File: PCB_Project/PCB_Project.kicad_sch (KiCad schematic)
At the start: 7 parts

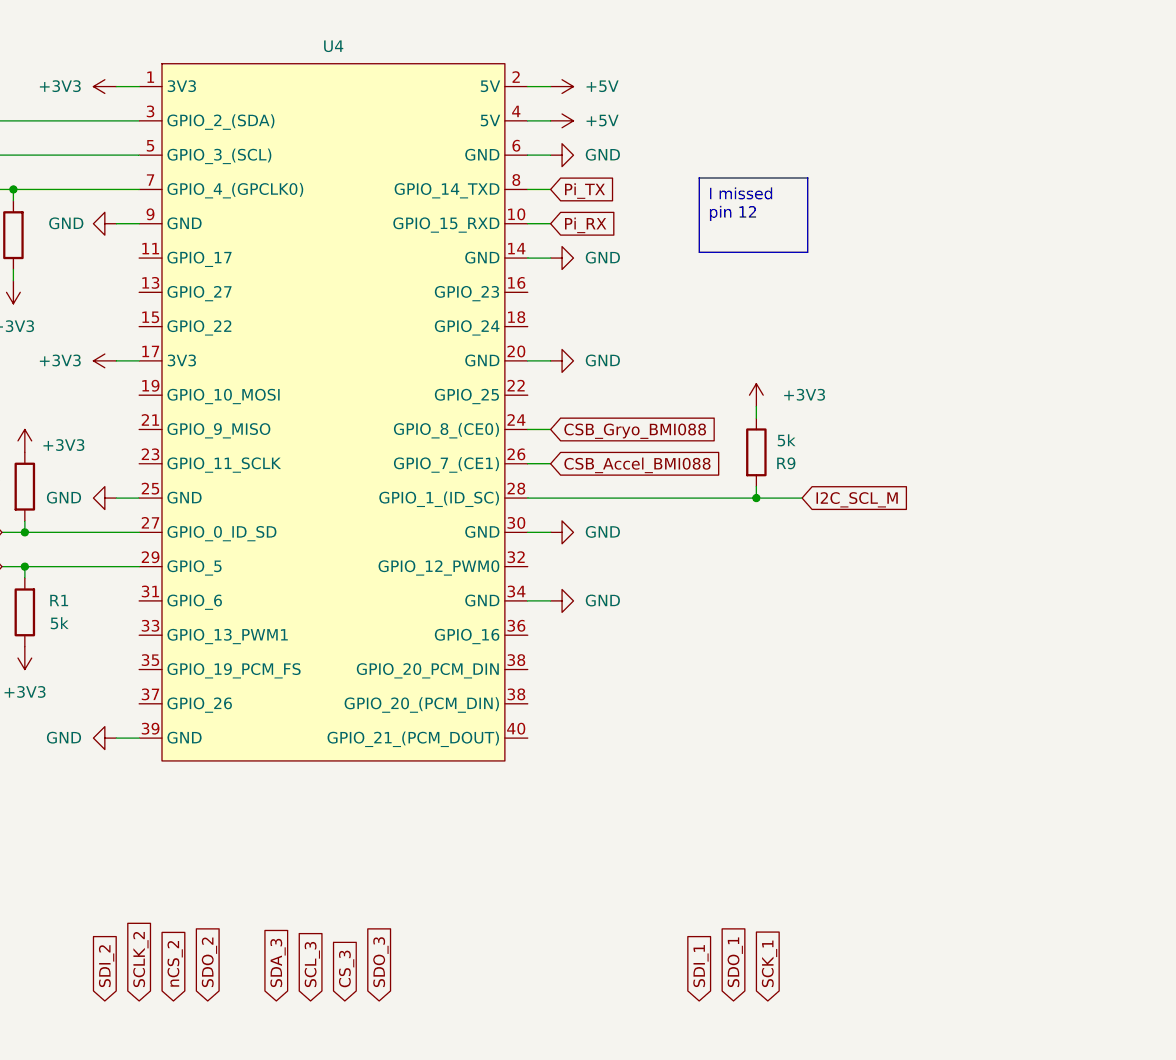
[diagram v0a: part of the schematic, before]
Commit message: more cleaning up and adding footprints
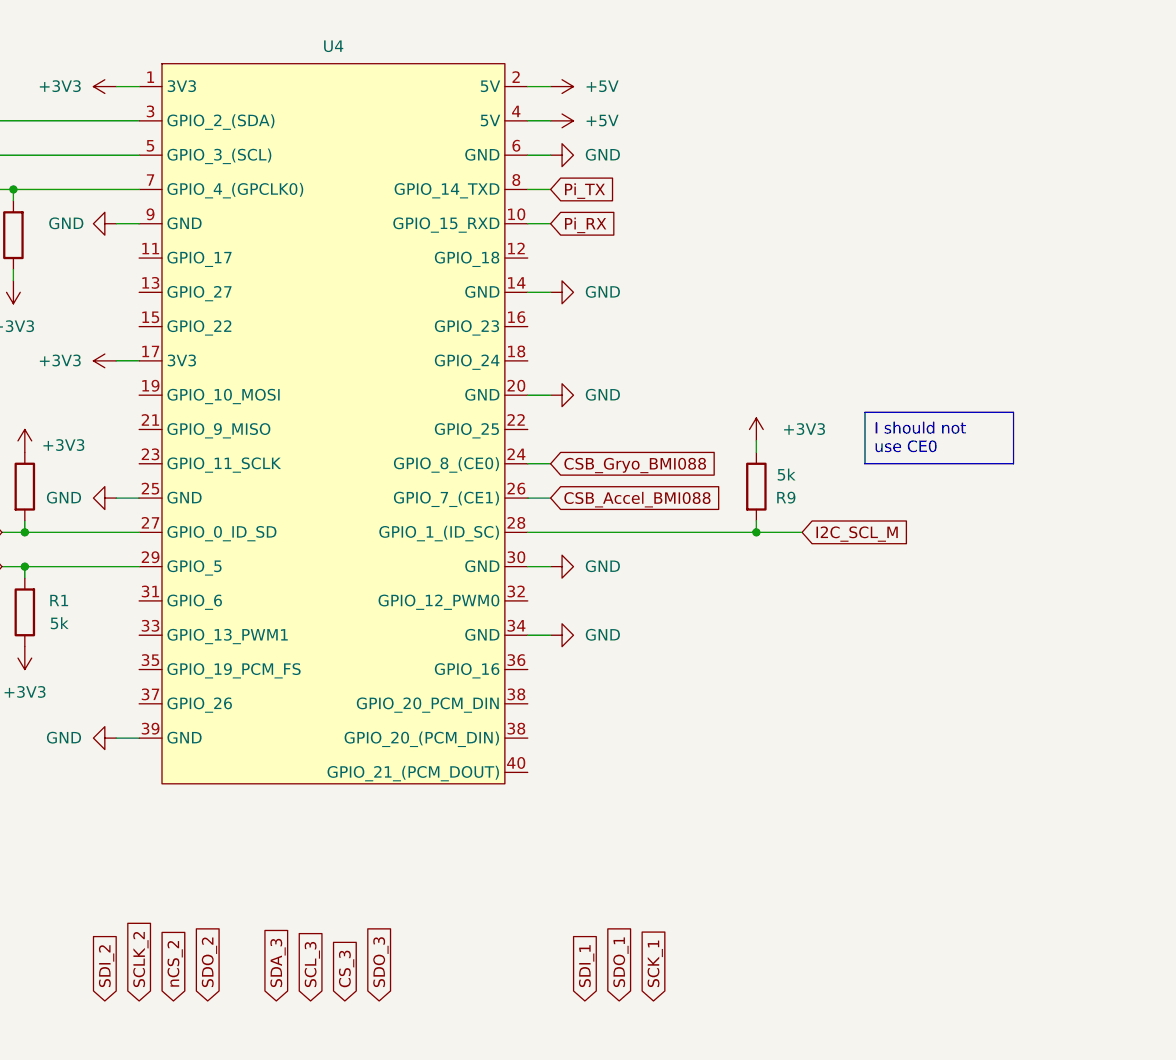
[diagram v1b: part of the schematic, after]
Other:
- moved on the sheet: R9

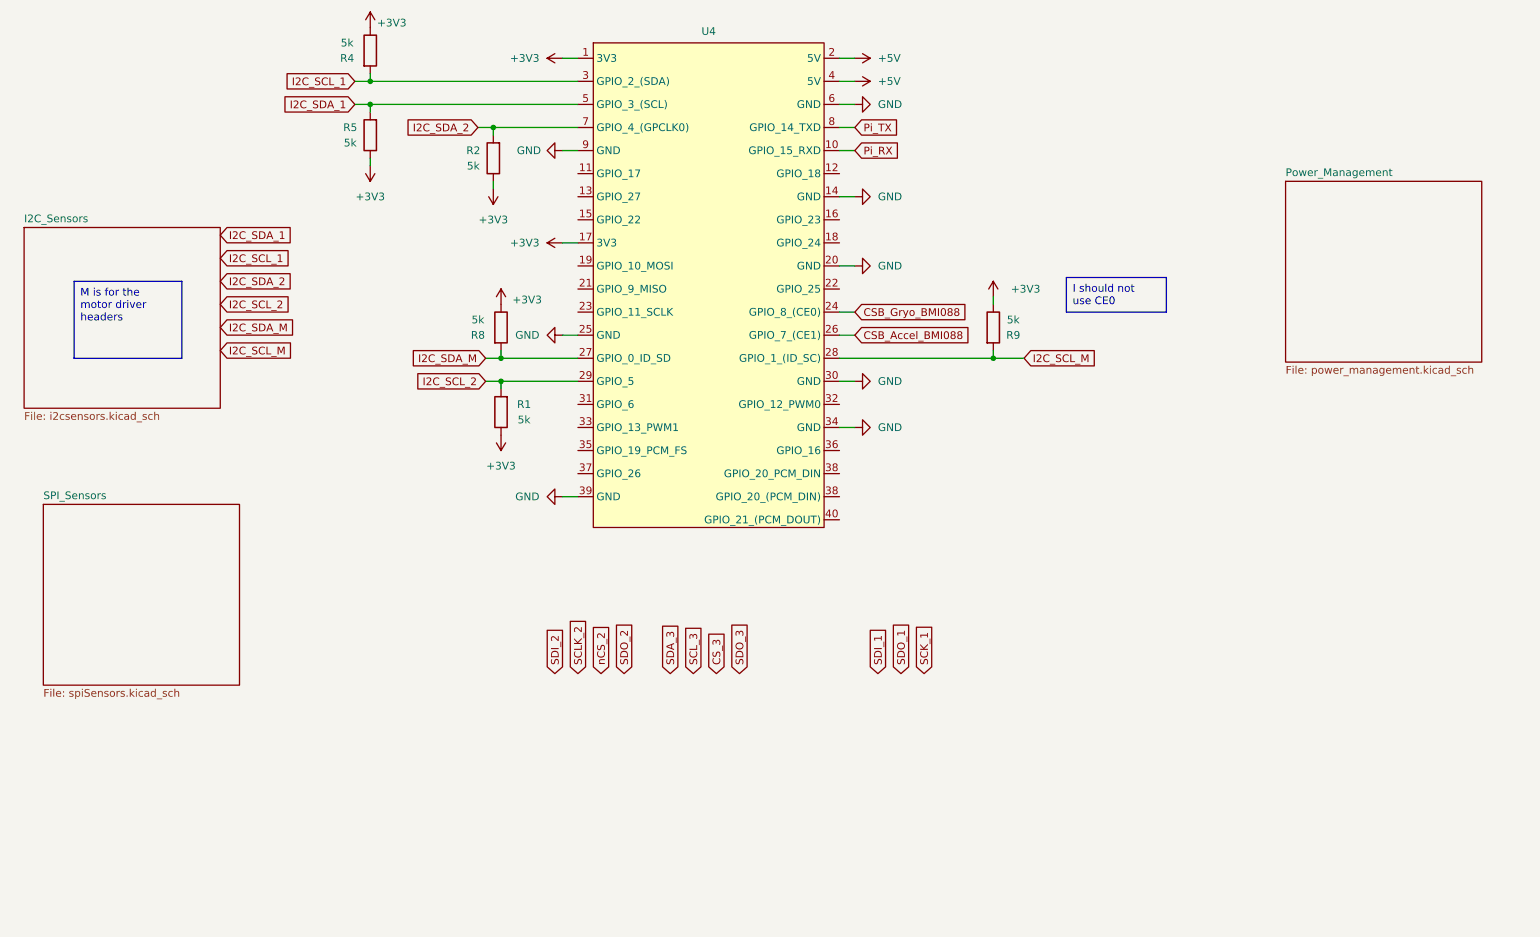
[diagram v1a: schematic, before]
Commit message: need to fix the one damn footprint
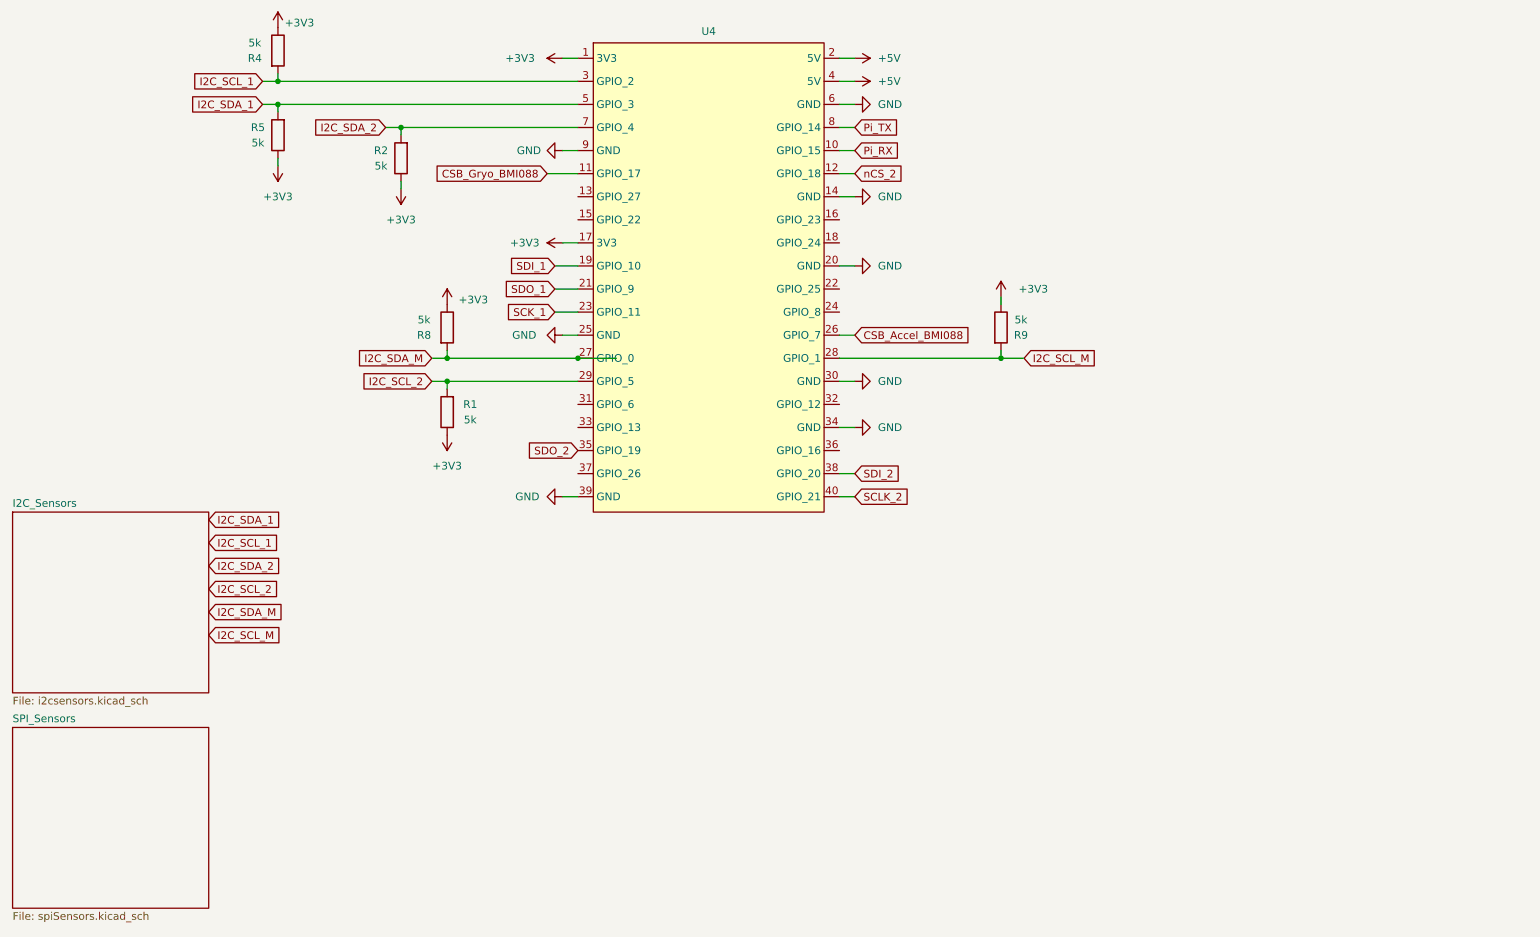
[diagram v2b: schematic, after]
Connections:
- net CSB_Gryo_BMI088: now also U4.11 (GPIO_17); no longer U4.24 (GPIO_8_(CE0))
- net SCK_1: now also U4.23 (GPIO_11)
- net SCLK_2: now also U4.40 (GPIO_21)
- net SDI_1: now also U4.19 (GPIO_10)
- net SDI_2: now also U4.38 (GPIO_20)
- net SDO_1: now also U4.21 (GPIO_9)
- net SDO_2: now also U4.35 (GPIO_19)
- net nCS_2: now also U4.12 (GPIO_18)
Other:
- removed sheet Power_Management
- moved on the sheet: R1, R2, R4, R5, R8, R9

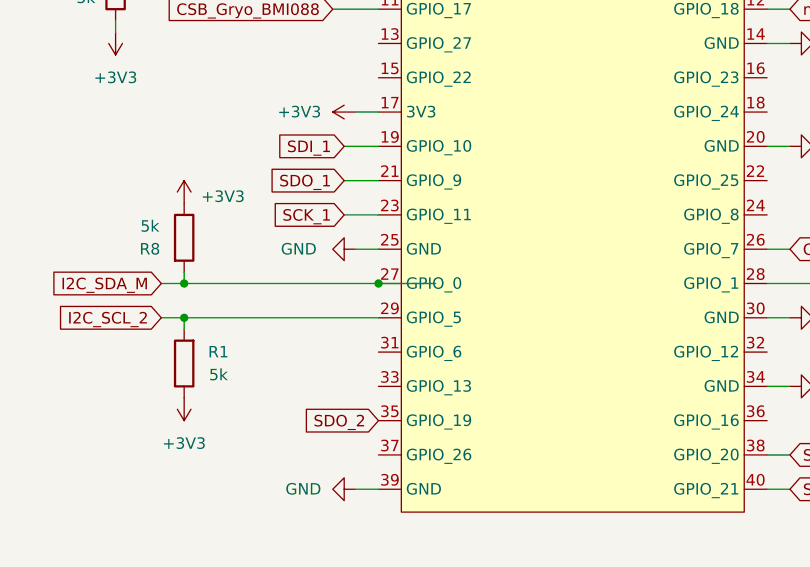
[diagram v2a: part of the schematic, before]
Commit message: re commit
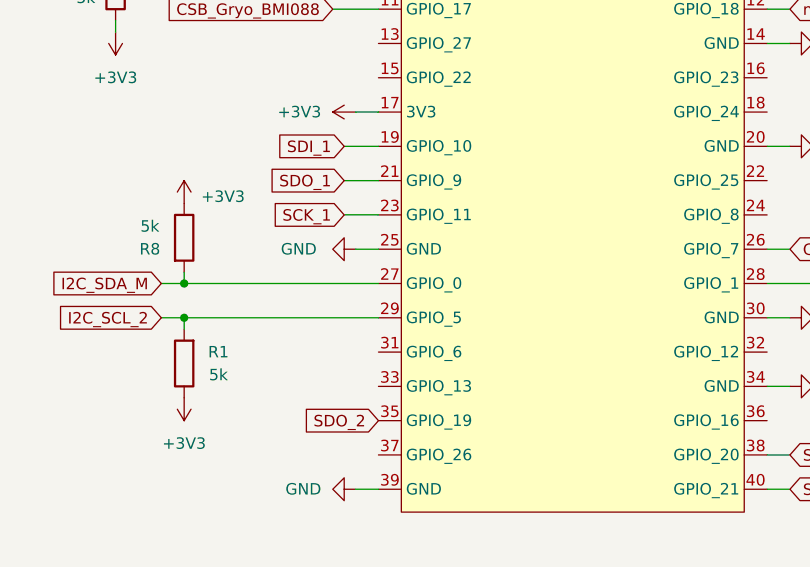
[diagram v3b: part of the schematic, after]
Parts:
- U4: footprint Connector_PinHeader_2.54mm:PinHeader_2x20_P2.54mm_Vertical -> Connector_PinSocket_2.54mm:PinSocket_2x20_P2.54mm_Vertical
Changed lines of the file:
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@@
-	)
-	(junction
-		(at 115.57 76.2)
-		(diameter 0)
-		(color 0 0 0 0)
 	)
 	(junction
@@
 	(wire
 		(pts
+			(xy 86.36 38.1) (xy 115.57 38.1)
+		)
+		(stroke
+			(width 0)
+			(type default)
+		)
+	)
+	(wire
+		(pts
+			(xy 161.29 41.91) (xy 158.75 41.91)
+		)
+		(stroke
+			(width 0)
+			(type default)
+		)
+	)
+	(wire
+		(pts
+			(xy 161.29 72.39) (xy 158.75 72.39)
+		)
+		(stroke
+			(width 0)
+			(type default)
+		)
+	)
+	(wire
+		(pts
+			(xy 185.42 76.2) (xy 189.23 76.2)
+		)
+		(stroke
+			(width 0)
+			(type default)
+		)
+	)
+	(wire
+		(pts
+			(xy 111.76 64.77) (xy 115.57 64.77)
+		)
+		(stroke
+			(width 0)
+			(type default)
+		)
+	)
+	(wire
+		(pts
+			(xy 115.57 72.39) (xy 113.03 72.39)
+		)
+		(stroke
+			(width 0)
+			(type default)
+		)
+	)
+	(wire
+		(pts
+			(xy 158.75 26.67) (xy 161.29 26.67)
+		)
+		(stroke
+			(width 0)
+			(type default)
+		)
+	)
+	(wire
+		(pts
+			(xy 158.75 60.96) (xy 161.29 60.96)
+		)
+		(stroke
+			(width 0)
+			(type default)
+		)
+	)
+	(wire
+		(pts
+			(xy 66.04 29.21) (xy 66.04 30.48)
+		)
+		(stroke
+			(width 0)
+			(type default)
+		)
+	)
+	(wire
+		(pts
+			(xy 66.04 30.48) (xy 115.57 30.48)
+		)
+		(stroke
+			(width 0)
+			(type default)
+		)
+	)
+	(wire
+		(pts
+			(xy 158.75 80.01) (xy 161.29 80.01)
+		)
+		(stroke
+			(width 0)
+			(type default)
+		)
+	)
+	(wire
+		(pts
+			(xy 66.04 35.56) (xy 66.04 34.29)
+		)
+		(stroke
+			(width 0)
+			(type default)
+		)
+	)
+	(wire
+		(pts
+			(xy 91.44 80.01) (xy 93.98 80.01)
+		)
+		(stroke
+			(width 0)
+			(type default)
+		)
+	)
+	(wire
+		(pts
+			(xy 161.29 99.06) (xy 158.75 99.06)
+		)
+		(stroke
+			(width 0)
+			(type default)
+		)
+	)
+	(wire
+		(pts
+			(xy 111.76 60.96) (xy 115.57 60.96)
+		)
+		(stroke
+			(width 0)
+			(type default)
+		)
+	)
+	(wire
+		(pts
+			(xy 83.82 38.1) (xy 86.36 38.1)
+		)
+		(stroke
+			(width 0)
+			(type default)
+		)
+	)
+	(wire
+		(pts
+			(xy 93.98 74.93) (xy 93.98 76.2)
+		)
+		(stroke
+			(width 0)
+			(type default)
+		)
+	)
+	(wire
+		(pts
+			(xy 158.75 38.1) (xy 161.29 38.1)
+		)
+		(stroke
+			(width 0)
+			(type default)
+		)
+	)
+	(wire
+		(pts
 			(xy 93.98 76.2) (xy 115.57 76.2)
 		)
@@
 	(wire
 		(pts
-			(xy 86.36 38.1) (xy 115.57 38.1)
-		)
-		(stroke
-			(width 0)
-			(type default)
-		)
-	)
-	(wire
-		(pts
-			(xy 161.29 41.91) (xy 158.75 41.91)
-		)
-		(stroke
-			(width 0)
-			(type default)
-		)
-	)
-	(wire
-		(pts
-			(xy 161.29 72.39) (xy 158.75 72.39)
-		)
-		(stroke
-			(width 0)
-			(type default)
-		)
-	)
-	(wire
-		(pts
-			(xy 185.42 76.2) (xy 189.23 76.2)
-		)
-		(stroke
-			(width 0)
-			(type default)
-		)
-	)
-	(wire
-		(pts
-			(xy 111.76 64.77) (xy 115.57 64.77)
-		)
-		(stroke
-			(width 0)
-			(type default)
-		)
-	)
-	(wire
-		(pts
-			(xy 115.57 72.39) (xy 113.03 72.39)
-		)
-		(stroke
-			(width 0)
-			(type default)
-		)
-	)
-	(wire
-		(pts
-			(xy 158.75 26.67) (xy 161.29 26.67)
-		)
-		(stroke
-			(width 0)
-			(type default)
-		)
-	)
-	(wire
-		(pts
-			(xy 158.75 60.96) (xy 161.29 60.96)
-		)
-		(stroke
-			(width 0)
-			(type default)
-		)
-	)
-	(wire
-		(pts
-			(xy 66.04 29.21) (xy 66.04 30.48)
-		)
-		(stroke
-			(width 0)
-			(type default)
-		)
-	)
-	(wire
-		(pts
-			(xy 66.04 30.48) (xy 115.57 30.48)
-		)
-		(stroke
-			(width 0)
-			(type default)
-		)
-	)
-	(wire
-		(pts
-			(xy 158.75 80.01) (xy 161.29 80.01)
-		)
-		(stroke
-			(width 0)
-			(type default)
-		)
-	)
-	(wire
-		(pts
-			(xy 66.04 35.56) (xy 66.04 34.29)
-		)
-		(stroke
-			(width 0)
-			(type default)
-		)
-	)
-	(wire
-		(pts
-			(xy 91.44 80.01) (xy 93.98 80.01)
-		)
-		(stroke
-			(width 0)
-			(type default)
-		)
-	)
-	(wire
-		(pts
-			(xy 161.29 99.06) (xy 158.75 99.06)
-		)
-		(stroke
-			(width 0)
-			(type default)
-		)
-	)
-	(wire
-		(pts
-			(xy 111.76 60.96) (xy 115.57 60.96)
-		)
-		(stroke
-			(width 0)
-			(type default)
-		)
-	)
-	(wire
-		(pts
-			(xy 83.82 38.1) (xy 86.36 38.1)
-		)
-		(stroke
-			(width 0)
-			(type default)
-		)
-	)
-	(wire
-		(pts
-			(xy 93.98 74.93) (xy 93.98 76.2)
-		)
-		(stroke
-			(width 0)
-			(type default)
-		)
-	)
-	(wire
-		(pts
-			(xy 158.75 38.1) (xy 161.29 38.1)
-		)
-		(stroke
-			(width 0)
-			(type default)
-		)
-	)
-	(wire
-		(pts
 			(xy 86.36 46.99) (xy 86.36 48.26)
 		)
@@
 		(pts
 			(xy 113.03 26.67) (xy 115.57 26.67)
-		)
-		(stroke
-			(width 0)
-			(type default)
-		)
-	)
-	(wire
-		(pts
-			(xy 121.92 76.2) (xy 115.57 76.2)
 		)
 		(stroke
@@
 			)
 		)
-		(property "Footprint" "Connector_PinHeader_2.54mm:PinHeader_2x20_P2.54mm_Vertical"
+		(property "Footprint" "Connector_PinSocket_2.54mm:PinSocket_2x20_P2.54mm_Vertical"
 			(at 120.65 25.4 0)
 			(effects
